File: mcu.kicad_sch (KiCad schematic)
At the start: 22 parts, among them J1 USB_C_Receptacle_USB2.0_16P, SW1 SW_Push, U1 ESP32-S3-MINI-1U, U4 HLK-10M05, U6 TLV62569DBV

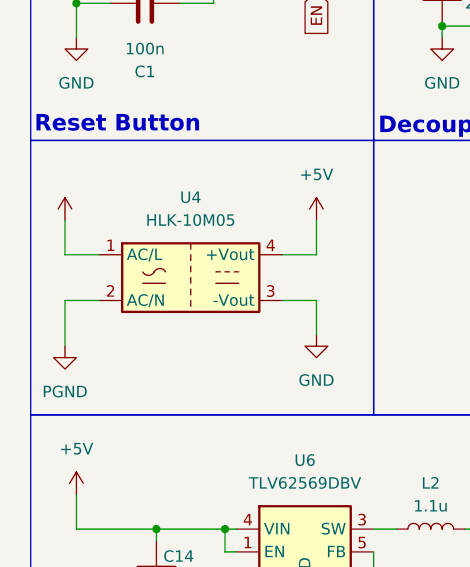
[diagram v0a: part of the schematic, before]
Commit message: relay connections
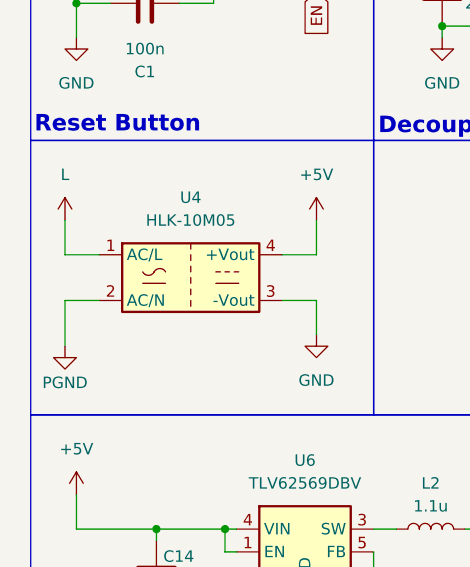
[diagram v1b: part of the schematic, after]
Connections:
- net L: now reaches U4.1 (AC/L)
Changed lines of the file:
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@@
-	)
-	(symbol
-		(lib_id "power:+3.3V")
-		(at 16.51 129.54 0)
-		(unit 1)
-		(body_style 1)
-		(exclude_from_sim no)
-		(in_bom yes)
-		(on_board yes)
-		(in_pos_files yes)
-		(dnp no)
-		(fields_autoplaced yes)
-		(property "Reference" "#PWR033"
-			(at 16.51 133.35 0)
-			(hide yes)
-			(show_name no)
-			(do_not_autoplace no)
-			(effects
-				(font
-					(size 1.27 1.27)
-				)
-			)
-		)
-		(property "Value" ""
-			(at 16.51 124.46 0)
-			(show_name no)
-			(do_not_autoplace no)
-			(effects
-				(font
-					(size 1.27 1.27)
-				)
-			)
-		)
-		(property "Footprint" "Package_DFN_QFN:Diodes_UDFN3810-9_TYPE_B"
-			(at 16.51 129.54 0)
-			(hide yes)
-			(show_name no)
-			(do_not_autoplace no)
-			(effects
-				(font
-					(size 1.27 1.27)
-				)
-			)
-		)
-		(property "Datasheet" ""
-			(at 16.51 129.54 0)
-			(hide yes)
-			(show_name no)
-			(do_not_autoplace no)
-			(effects
-				(font
-					(size 1.27 1.27)
-				)
-			)
-		)
-		(property "Description" "Power symbol creates a global label with name \"+3.3V\""
-			(at 16.51 129.54 0)
-			(hide yes)
-			(show_name no)
-			(do_not_autoplace no)
-			(effects
-				(font
-					(size 1.27 1.27)
-				)
-			)
-		)
-		(pin "1"
-		)
-		(instances
-			(project "smart_supply"
-				(path "/487ef637-7a03-4925-80c1-798e0c6f0bbd/f9380e13-e191-4828-b42d-2cc7f479b711"
-					(reference "#PWR033")
-					(unit 1)
-				)
-			)
-		)
 	)
 	(symbol
@@
 	)
 	(symbol
+		(lib_id "power:+3.3V")
+		(at 16.51 129.54 0)
+		(unit 1)
+		(body_style 1)
+		(exclude_from_sim no)
+		(in_bom yes)
+		(on_board yes)
+		(in_pos_files yes)
+		(dnp no)
+		(fields_autoplaced yes)
+		(property "Reference" "#PWR049"
+			(at 16.51 133.35 0)
+			(hide yes)
+			(show_name no)
+			(do_not_autoplace no)
+			(effects
+				(font
+					(size 1.27 1.27)
+				)
+			)
+		)
+		(property "Value" "L"
+			(at 16.51 124.46 0)
+			(show_name no)
+			(do_not_autoplace no)
+			(effects
+				(font
+					(size 1.27 1.27)
+				)
+			)
+		)
+		(property "Footprint" "Package_DFN_QFN:Diodes_UDFN3810-9_TYPE_B"
+			(at 16.51 129.54 0)
+			(hide yes)
+			(show_name no)
+			(do_not_autoplace no)
+			(effects
+				(font
+					(size 1.27 1.27)
+				)
+			)
+		)
+		(property "Datasheet" ""
+			(at 16.51 129.54 0)
+			(hide yes)
+			(show_name no)
+			(do_not_autoplace no)
+			(effects
+				(font
+					(size 1.27 1.27)
+				)
+			)
+		)
+		(property "Description" "Power symbol creates a global label with name \"+3.3V\""
+			(at 16.51 129.54 0)
+			(hide yes)
+			(show_name no)
+			(do_not_autoplace no)
+			(effects
+				(font
+					(size 1.27 1.27)
+				)
+			)
+		)
+		(pin "1"
+		)
+		(instances
+			(project "smart_supply"
+				(path "/487ef637-7a03-4925-80c1-798e0c6f0bbd/f9380e13-e191-4828-b42d-2cc7f479b711"
+					(reference "#PWR049")
+					(unit 1)
+				)
+			)
+		)
+	)
+	(symbol
 		(lib_id "Converter_ACDC:HLK-10M05")
 		(at 30.48 135.89 0)
@@
 		(in_pos_files yes)
 		(dnp no)
-		(fields_autoplaced yes)
 		(property "Reference" "#PWR034"
 			(at 16.51 149.86 0)
@@
 		)
 		(property "Value" "PGND"
-			(at 16.51 148.59 0)
-			(show_name no)
-			(do_not_autoplace no)
+			(at 16.51 147.574 0)
+			(show_name no)
+			(do_not_autoplace no)
